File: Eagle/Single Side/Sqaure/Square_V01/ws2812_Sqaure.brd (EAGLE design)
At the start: 25.4 x 25.4 mm, 10 parts

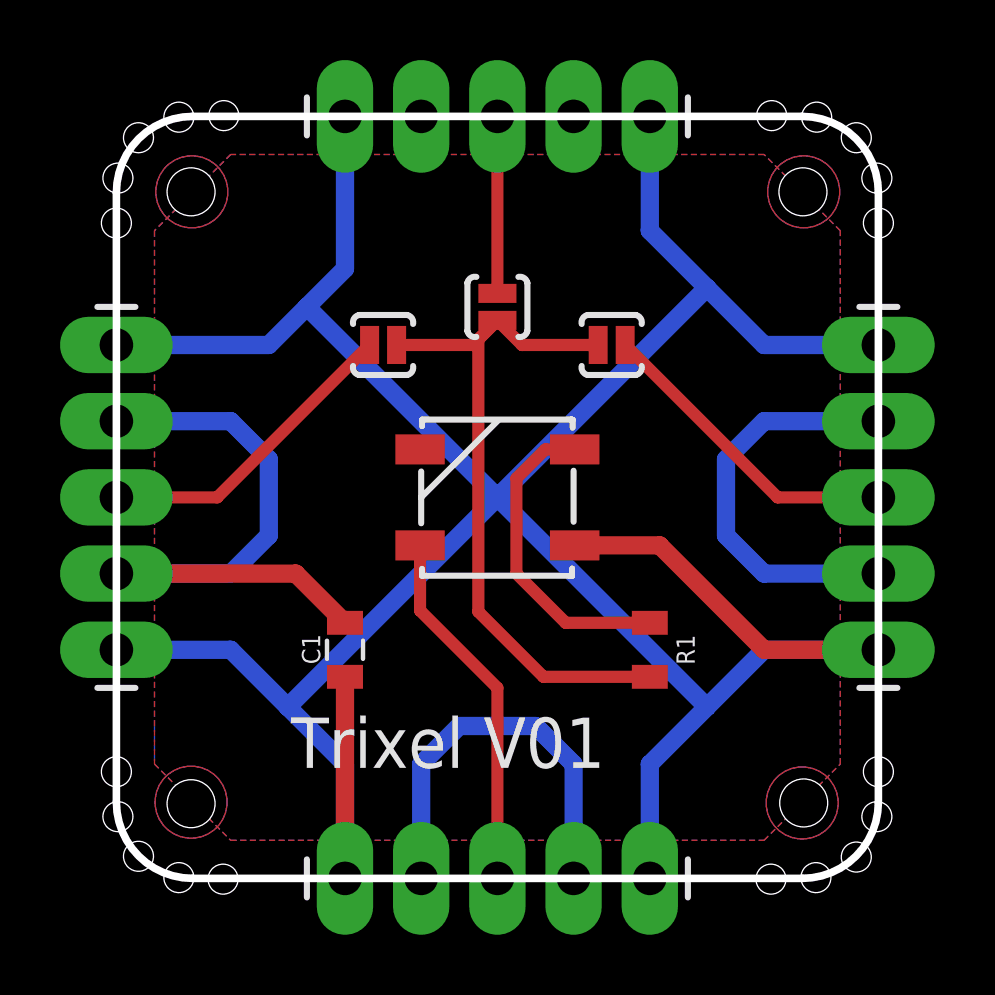
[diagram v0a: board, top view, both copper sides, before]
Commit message: Latest large panel designes
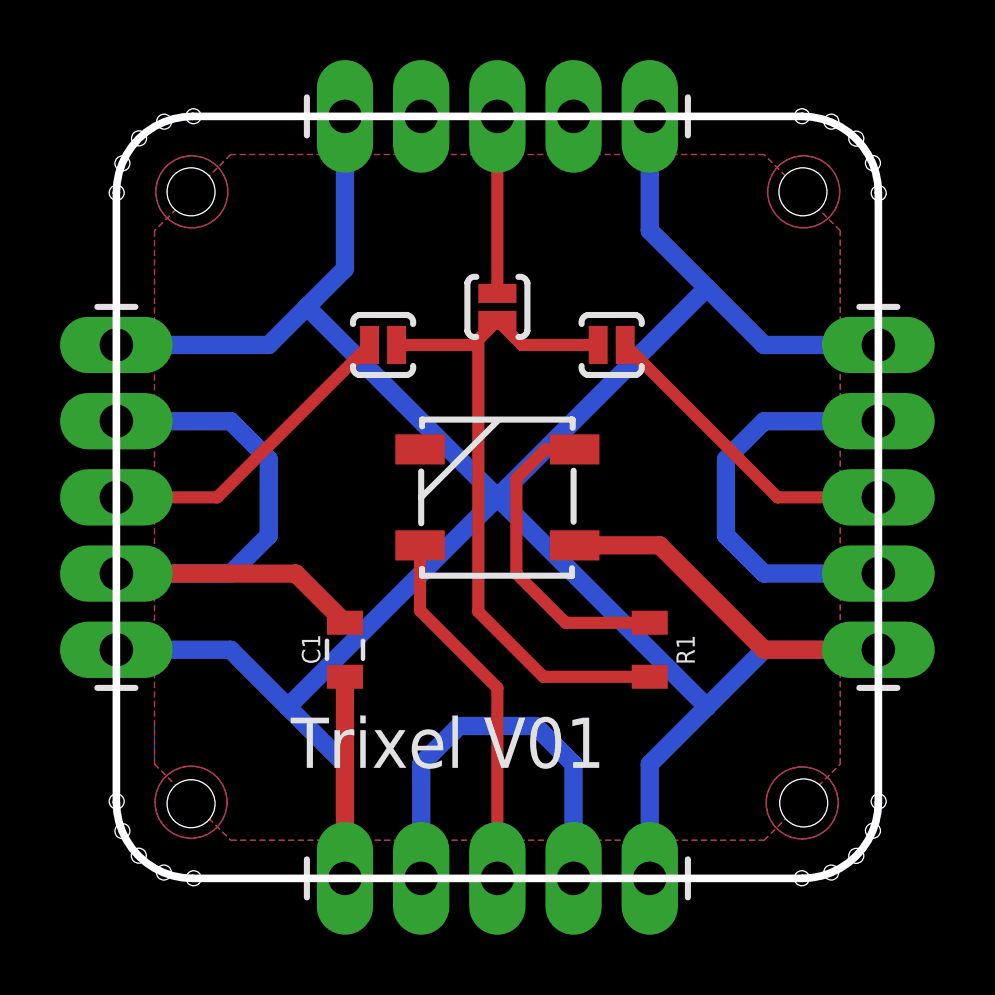
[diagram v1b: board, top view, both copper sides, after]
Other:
- board text added: "C1"
- board text added: "R1"
